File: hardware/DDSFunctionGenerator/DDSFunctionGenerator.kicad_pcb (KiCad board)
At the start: 2 copper layers, 100 x 80 mm, 137 parts, among them J1 Conn_Coaxial, J2 USB_B_Micro, J3 Conn_Coaxial, J4 Conn_Coaxial, Q1 Q_NPN_BEC, Q2 Q_NPN_BEC, Q3 Q_NPN_BEC, Q4 BC859, Q5 BC848, SW1 Rotary_Encoder_Switch, T1 Transformer_1P_1S, U1 TC1107-3.3VOA, U10 74HCT1G86, U2 L7805, U3 L7805, U4 AD9832, U5 STM32F030K6Tx, U6 FT200XD, U7 AD8325, U8 MCP3425A0T-ECH, U9 LM358, X1 XO91, Y1 Crystal

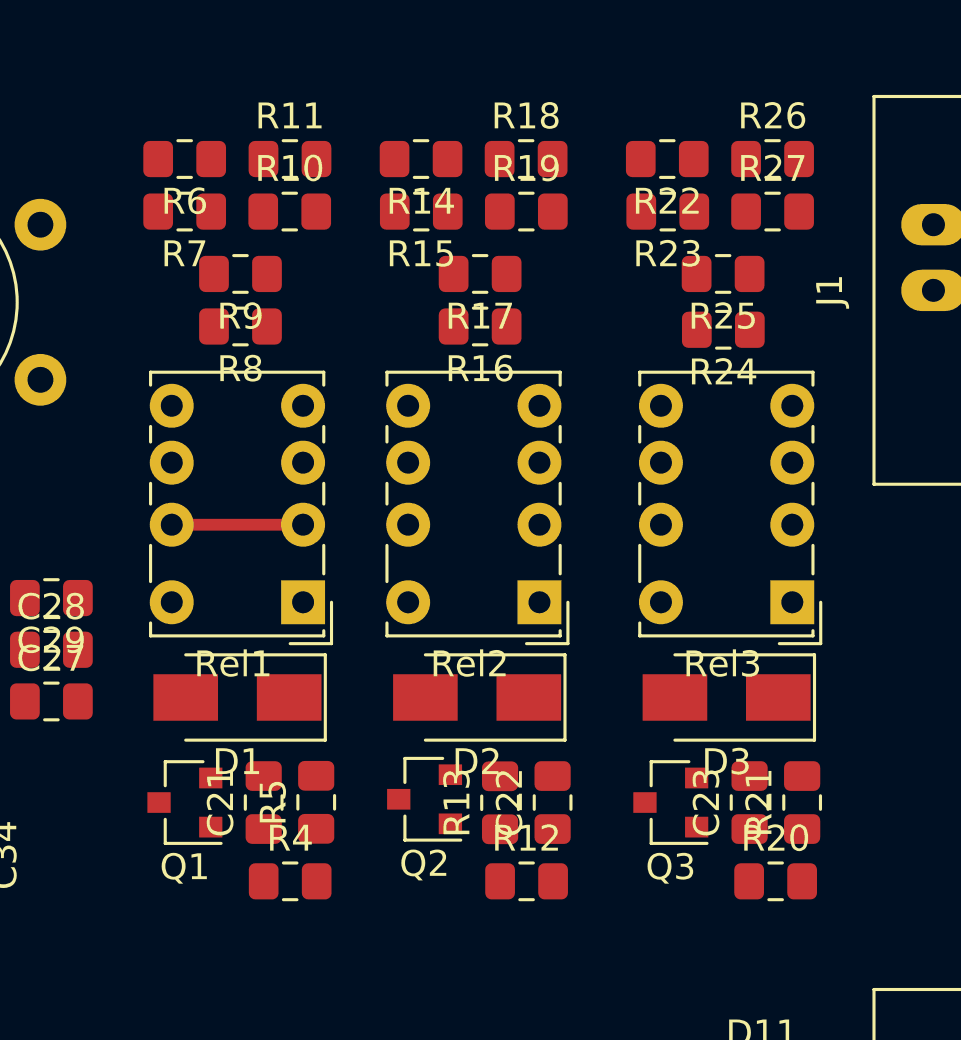
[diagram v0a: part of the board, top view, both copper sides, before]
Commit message: update to recent kicad version
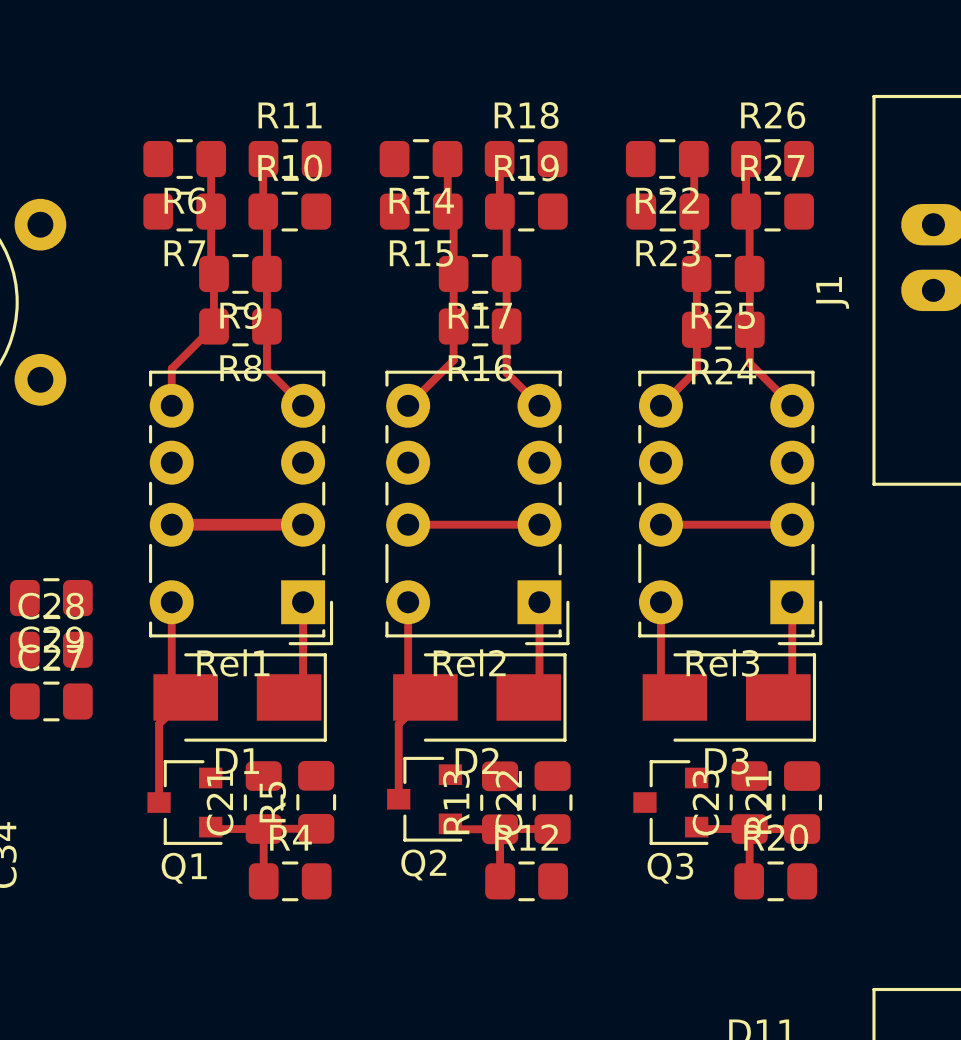
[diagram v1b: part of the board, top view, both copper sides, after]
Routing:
- net +9V: track 0.00 -> 11.7 mm
- net Net-(R14-Pad1): track 0.00 -> 10.4 mm
- net Net-(R24-Pad1): track 0.00 -> 10.3 mm
- net Net-(R6-Pad1): track 0.00 -> 10.3 mm
- net Net-(R10-Pad1): track 0.00 -> 10.2 mm
- net Net-(R16-Pad1): track 0.00 -> 10.2 mm
- net Net-(R22-Pad1): track 0.00 -> 10.2 mm
- net Net-(D1-Pad2): track 0.00 -> 8.40 mm
- net Net-(D2-Pad2): track 0.00 -> 8.32 mm
- net Net-(C23-Pad1): track 0.00 -> 6.14 mm
- net Net-(C21-Pad1): track 0.00 -> 6.14 mm
- net Net-(C22-Pad1): track 0.00 -> 6.06 mm
- net Net-(Rel3-Pad2): track 0.00 -> 5.08 mm
- net Net-(Rel2-Pad2): track 0.00 -> 5.08 mm
- net Net-(D3-Pad2): track 0.00 -> 3.91 mm
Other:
- net class Default: trace_width 0.25 -> 0.3048
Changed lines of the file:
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@@
-(kicad_pcb (version 20171130) (host pcbnew "(5.1.2)-1")
+(kicad_pcb (version 20171130) (host pcbnew 5.0.2-bee76a0~70~ubuntu18.04.1)
   (general
     (thickness 1.6)
     (drawings 5)
-    (tracks 1)
+    (tracks 76)
     (zones 0)
     (modules 137)
@@
   )
   (setup
-    (last_trace_width 0.25)
+    (last_trace_width 0.3048)
     (user_trace_width 0.4572)
     (trace_clearance 0.2)
@@
     (zone_45_only no)
     (trace_min 0.2)
+    (segment_width 0.2)
+    (edge_width 0.05)
     (via_size 0.8)
     (via_drill 0.4)
@@
     (uvia_min_size 0.2)
     (uvia_min_drill 0.1)
-    (edge_width 0.05)
-    (segment_width 0.2)
     (pcb_text_width 0.3)
     (pcb_text_size 1.5 1.5)
@@
   (net_class Default "This is the default net class."
     (clearance 0.2)
-    (trace_width 0.25)
+    (trace_width 0.3048)
     (via_dia 0.8)
     (via_drill 0.4)
@@
   (gr_line (start 150 60) (end 150 140) (layer Edge.Cuts) (width 0.05))
   (gr_line (start 50 60) (end 150 60) (layer Edge.Cuts) (width 0.05))
+  (segment (start 131.699 86.836) (end 131.159 87.376) (width 0.3048) (layer F.Cu) (net 1))
+  (segment (start 131.699 83.693) (end 131.699 86.836) (width 0.3048) (layer F.Cu) (net 1))
+  (segment (start 121.92 86.963) (end 121.507 87.376) (width 0.3048) (layer F.Cu) (net 1))
+  (segment (start 121.92 83.693) (end 121.92 86.963) (width 0.3048) (layer F.Cu) (net 1))
+  (segment (start 112.776 86.836) (end 112.236 87.376) (width 0.3048) (layer F.Cu) (net 1))
+  (segment (start 112.776 83.693) (end 112.776 86.836) (width 0.3048) (layer F.Cu) (net 1))
+  (segment (start 107.696 86.836) (end 108.236 87.376) (width 0.3048) (layer F.Cu) (net 3))
+  (segment (start 107.696 83.693) (end 107.696 86.836) (width 0.3048) (layer F.Cu) (net 3))
+  (segment (start 107.204 88.408) (end 108.236 87.376) (width 0.3048) (layer F.Cu) (net 3))
+  (segment (start 107.204 91.44) (end 107.204 88.408) (width 0.3048) (layer F.Cu) (net 3))
+  (segment (start 116.84 86.709) (end 117.507 87.376) (width 0.3048) (layer F.Cu) (net 4))
+  (segment (start 116.84 83.693) (end 116.84 86.709) (width 0.3048) (layer F.Cu) (net 4))
+  (segment (start 116.475 88.408) (end 117.507 87.376) (width 0.3048) (layer F.Cu) (net 4))
+  (segment (start 116.475 91.313) (end 116.475 88.408) (width 0.3048) (layer F.Cu) (net 4))
+  (segment (start 126.619 86.836) (end 127.159 87.376) (width 0.3048) (layer F.Cu) (net 6))
+  (segment (start 126.619 83.693) (end 126.619 86.836) (width 0.3048) (layer F.Cu) (net 6))
+  (segment (start 111.261 92.456) (end 111.252 92.465) (width 0.3048) (layer F.Cu) (net 26))
+  (segment (start 113.284 92.456) (end 111.261 92.456) (width 0.3048) (layer F.Cu) (net 26))
+  (segment (start 111.252 92.465) (end 111.252 94.488) (width 0.3048) (layer F.Cu) (net 26))
+  (segment (start 109.279 92.465) (end 109.204 92.39) (width 0.3048) (layer F.Cu) (net 26))
+  (segment (start 111.252 92.465) (end 109.279 92.465) (width 0.3048) (layer F.Cu) (net 26))
+  (segment (start 120.405 92.465) (end 120.396 92.474) (width 0.3048) (layer F.Cu) (net 27))
+  (segment (start 122.428 92.465) (end 120.405 92.465) (width 0.3048) (layer F.Cu) (net 27))
+  (segment (start 120.396 92.474) (end 120.396 94.488) (width 0.3048) (layer F.Cu) (net 27))
+  (segment (start 118.686 92.474) (end 118.475 92.263) (width 0.3048) (layer F.Cu) (net 27))
+  (segment (start 120.396 92.474) (end 118.686 92.474) (width 0.3048) (layer F.Cu) (net 27))
+  (segment (start 132.08 92.465) (end 130.048 92.465) (width 0.3048) (layer F.Cu) (net 28))
+  (segment (start 130.048 94.47) (end 130.03 94.488) (width 0.3048) (layer F.Cu) (net 28))
+  (segment (start 130.048 92.465) (end 130.048 94.47) (width 0.3048) (layer F.Cu) (net 28))
+  (segment (start 128.075 92.465) (end 128 92.39) (width 0.3048) (layer F.Cu) (net 28))
+  (segment (start 130.048 92.465) (end 128.075 92.465) (width 0.3048) (layer F.Cu) (net 28))
+  (segment (start 107.696 74.658) (end 107.696 76.093) (width 0.3048) (layer F.Cu) (net 29))
+  (segment (start 109.329 73.025) (end 107.696 74.658) (width 0.3048) (layer F.Cu) (net 29))
+  (segment (start 109.22 66.548) (end 109.22 68.58) (width 0.3048) (layer F.Cu) (net 29))
+  (segment (start 109.22 70.884) (end 109.329 70.993) (width 0.3048) (layer F.Cu) (net 29))
+  (segment (start 109.22 68.58) (end 109.22 70.884) (width 0.3048) (layer F.Cu) (net 29))
+  (segment (start 109.329 70.993) (end 109.329 73.025) (width 0.3048) (layer F.Cu) (net 29))
+  (segment (start 111.379 74.696) (end 112.776 76.093) (width 0.3048) (layer F.Cu) (net 30))
+  (segment (start 111.379 73.025) (end 111.379 74.696) (width 0.3048) (layer F.Cu) (net 30))
+  (segment (start 111.379 73.025) (end 111.379 70.993) (width 0.3048) (layer F.Cu) (net 30))
+  (segment (start 111.379 68.725) (end 111.234 68.58) (width 0.3048) (layer F.Cu) (net 30))
+  (segment (start 111.379 70.993) (end 111.379 68.725) (width 0.3048) (layer F.Cu) (net 30))
+  (segment (start 111.234 66.557) (end 111.243 66.548) (width 0.3048) (layer F.Cu) (net 30))
+  (segment (start 111.234 68.58) (end 111.234 66.557) (width 0.3048) (layer F.Cu) (net 30))
   (segment (start 107.823 80.693) (end 112.903 80.693) (width 0.4572) (layer F.Cu) (net 34))
+  (segment (start 118.6 73.025) (end 118.6 70.993) (width 0.3048) (layer F.Cu) (net 35))
+  (segment (start 118.6 68.807) (end 118.373 68.58) (width 0.3048) (layer F.Cu) (net 35))
+  (segment (start 118.6 70.993) (end 118.6 68.807) (width 0.3048) (layer F.Cu) (net 35))
+  (segment (start 118.373 66.557) (end 118.364 66.548) (width 0.3048) (layer F.Cu) (net 35))
+  (segment (start 118.373 68.58) (end 118.373 66.557) (width 0.3048) (layer F.Cu) (net 35))
+  (segment (start 118.6 74.333) (end 116.84 76.093) (width 0.3048) (layer F.Cu) (net 35))
+  (segment (start 118.6 73.025) (end 118.6 74.333) (width 0.3048) (layer F.Cu) (net 35))
+  (segment (start 120.65 73.025) (end 120.65 70.993) (width 0.3048) (layer F.Cu) (net 36))
+  (segment (start 120.65 68.843) (end 120.387 68.58) (width 0.3048) (layer F.Cu) (net 36))
+  (segment (start 120.65 70.993) (end 120.65 68.843) (width 0.3048) (layer F.Cu) (net 36))
+  (segment (start 120.387 66.557) (end 120.378 66.548) (width 0.3048) (layer F.Cu) (net 36))
+  (segment (start 120.387 68.58) (end 120.387 66.557) (width 0.3048) (layer F.Cu) (net 36))
+  (segment (start 120.65 74.823) (end 121.92 76.093) (width 0.3048) (layer F.Cu) (net 36))
+  (segment (start 120.65 73.025) (end 120.65 74.823) (width 0.3048) (layer F.Cu) (net 36))
+  (segment (start 116.84 80.693) (end 121.92 80.693) (width 0.3048) (layer F.Cu) (net 37))
+  (segment (start 128.007 74.705) (end 126.619 76.093) (width 0.3048) (layer F.Cu) (net 38))
+  (segment (start 128.007 73.152) (end 128.007 74.705) (width 0.3048) (layer F.Cu) (net 38))
+  (segment (start 128.007 71.002) (end 127.998 70.993) (width 0.3048) (layer F.Cu) (net 38))
+  (segment (start 128.007 73.152) (end 128.007 71.002) (width 0.3048) (layer F.Cu) (net 38))
+  (segment (start 127.998 68.671) (end 127.907 68.58) (width 0.3048) (layer F.Cu) (net 38))
+  (segment (start 127.998 70.993) (end 127.998 68.671) (width 0.3048) (layer F.Cu) (net 38))
+  (segment (start 127.907 66.566) (end 127.889 66.548) (width 0.3048) (layer F.Cu) (net 38))
+  (segment (start 127.907 68.58) (end 127.907 66.566) (width 0.3048) (layer F.Cu) (net 38))
+  (segment (start 130.057 74.451) (end 131.699 76.093) (width 0.3048) (layer F.Cu) (net 39))
+  (segment (start 130.057 73.152) (end 130.057 74.451) (width 0.3048) (layer F.Cu) (net 39))
+  (segment (start 130.057 71.002) (end 130.048 70.993) (width 0.3048) (layer F.Cu) (net 39))
+  (segment (start 130.057 73.152) (end 130.057 71.002) (width 0.3048) (layer F.Cu) (net 39))
+  (segment (start 130.048 68.716) (end 129.912 68.58) (width 0.3048) (layer F.Cu) (net 39))
+  (segment (start 130.048 70.993) (end 130.048 68.716) (width 0.3048) (layer F.Cu) (net 39))
+  (segment (start 129.912 68.58) (end 129.912 66.548) (width 0.3048) (layer F.Cu) (net 39))
+  (segment (start 126.619 80.693) (end 131.699 80.693) (width 0.3048) (layer F.Cu) (net 40))
   (zone (net 7) (net_name GND) (layer F.Cu) (hatch edge 0.508)
     (connect_pads (clearance 0.508))
